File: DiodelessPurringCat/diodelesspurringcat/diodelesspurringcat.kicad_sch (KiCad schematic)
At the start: 21 parts, among them J1 ScreenL, U1 ProMicro-kbd

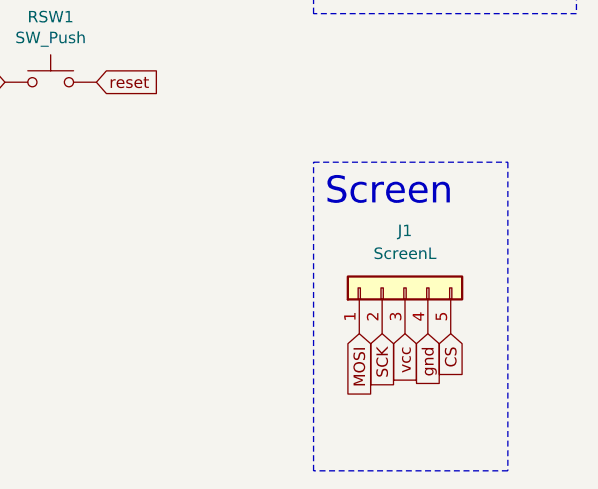
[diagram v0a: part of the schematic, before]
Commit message: trying to make a reversible nice view
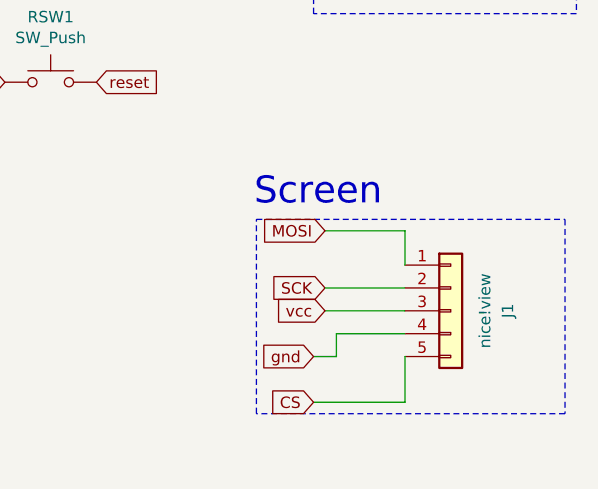
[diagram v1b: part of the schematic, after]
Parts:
- 0/9, 1/8, 10/19, 11/18, 12/17, 13/16, 14/15, 2/7, 20/25, 21/24, 22/23, 26/29, 27/28, 3/6, 4/5: footprint keyswitches:Kailh_socket_PG1350_reversible -> chelming-kbd:choc_v1_hotswap_reversible_no_extras
- J1: value ScreenL -> nice!view; footprint Connector_PinHeader_2.54mm:PinHeader_1x05_P2.54mm_Vertical -> chelming-kbd:nice-view_reversible
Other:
- moved on the sheet: J1
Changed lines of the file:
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@@
 	(polyline
 		(pts
-			(xy 227.33 124.46) (xy 205.74 124.46)
+			(xy 199.39 118.11) (xy 199.39 96.52)
 		)
 		(stroke
@@
 		)
 	)
+	(wire
+		(pts
+			(xy 205.74 111.76) (xy 208.28 111.76)
+		)
+		(stroke
+			(width 0)
+			(type default)
+		)
+	)
+	(wire
+		(pts
+			(xy 207.01 104.14) (xy 215.9 104.14)
+		)
+		(stroke
+			(width 0)
+			(type default)
+		)
+	)
+	(wire
+		(pts
+			(xy 205.74 116.84) (xy 215.9 116.84)
+		)
+		(stroke
+			(width 0)
+			(type default)
+		)
+	)
+	(wire
+		(pts
+			(xy 215.9 97.79) (xy 215.9 101.6)
+		)
+		(stroke
+			(width 0)
+			(type default)
+		)
+	)
+	(wire
+		(pts
+			(xy 215.9 116.84) (xy 215.9 111.76)
+		)
+		(stroke
+			(width 0)
+			(type default)
+		)
+	)
 	(polyline
 		(pts
-			(xy 227.33 90.17) (xy 227.33 124.46)
+			(xy 233.68 118.11) (xy 199.39 118.11)
 		)
 		(stroke
@@
 	(polyline
 		(pts
-			(xy 205.74 124.46) (xy 205.74 90.17)
+			(xy 199.39 96.52) (xy 233.68 96.52)
 		)
 		(stroke
@@
 	(polyline
 		(pts
-			(xy 205.74 90.17) (xy 227.33 90.17)
+			(xy 233.68 96.52) (xy 233.68 118.11)
 		)
 		(stroke
@@
 		)
 	)
+	(wire
+		(pts
+			(xy 208.28 109.22) (xy 215.9 109.22)
+		)
+		(stroke
+			(width 0)
+			(type default)
+		)
+	)
+	(wire
+		(pts
+			(xy 207.01 106.68) (xy 215.9 106.68)
+		)
+		(stroke
+			(width 0)
+			(type default)
+		)
+	)
+	(wire
+		(pts
+			(xy 208.28 111.76) (xy 208.28 109.22)
+		)
+		(stroke
+			(width 0)
+			(type default)
+		)
+	)
 	(polyline
 		(pts
@@
 		)
 	)
+	(wire
+		(pts
+			(xy 207.01 97.79) (xy 215.9 97.79)
+		)
+		(stroke
+			(width 0)
+			(type default)
+		)
+	)
 	(polyline
 		(pts
@@
 	(text "Screen"
 		(exclude_from_sim no)
-		(at 207.01 95.25 0)
+		(at 199.136 95.25 0)
 		(effects
 			(font
@@
 	(global_label "gnd"
 		(shape input)
-		(at 218.44 109.22 270)
-		(fields_autoplaced yes)
-		(effects
-			(font
-				(size 1.27 1.27)
-			)
-			(justify right)
-		)
-		(property "Intersheetrefs" "${INTERSHEET_REFS}"
-			(at 218.3606 114.9913 90)
+		(at 205.74 111.76 180)
+		(fields_autoplaced yes)
+		(effects
+			(font
+				(size 1.27 1.27)
+			)
+			(justify right)
+		)
+		(property "Intersheetrefs" "${INTERSHEET_REFS}"
+			(at 199.962 111.76 0)
 			(effects
 				(font
@@
 	(global_label "CS"
 		(shape input)
-		(at 220.98 109.22 270)
-		(fields_autoplaced yes)
-		(effects
-			(font
-				(size 1.27 1.27)
-			)
-			(justify right)
-		)
-		(property "Intersheetrefs" "${INTERSHEET_REFS}"
-			(at 220.9006 114.0237 90)
+		(at 205.74 116.84 180)
+		(fields_autoplaced yes)
+		(effects
+			(font
+				(size 1.27 1.27)
+			)
+			(justify right)
+		)
+		(property "Intersheetrefs" "${INTERSHEET_REFS}"
+			(at 200.9295 116.84 0)
 			(effects
 				(font
@@
 	(global_label "vcc"
 		(shape input)
-		(at 215.9 109.22 270)
-		(fields_autoplaced yes)
-		(effects
-			(font
-				(size 1.27 1.27)
-			)
-			(justify right)
-		)
-		(property "Intersheetrefs" "${INTERSHEET_REFS}"
-			(at 215.8206 114.689 90)
+		(at 207.01 106.68 180)
+		(fields_autoplaced yes)
+		(effects
+			(font
+				(size 1.27 1.27)
+			)
+			(justify right)
+		)
+		(property "Intersheetrefs" "${INTERSHEET_REFS}"
+			(at 201.5342 106.68 0)
 			(effects
 				(font
@@
 	(global_label "SCK"
 		(shape input)
-		(at 213.36 109.22 270)
-		(fields_autoplaced yes)
-		(effects
-			(font
-				(size 1.27 1.27)
-			)
-			(justify right)
-		)
-		(property "Intersheetrefs" "${INTERSHEET_REFS}"
-			(at 213.2806 115.2937 90)
+		(at 207.01 104.14 180)
+		(fields_autoplaced yes)
+		(effects
+			(font
+				(size 1.27 1.27)
+			)
+			(justify right)
+		)
+		(property "Intersheetrefs" "${INTERSHEET_REFS}"
+			(at 200.9295 104.14 0)
 			(effects
 				(font
@@
 	(global_label "MOSI"
 		(shape input)
-		(at 210.82 109.22 270)
-		(fields_autoplaced yes)
-		(effects
-			(font
-				(size 1.27 1.27)
-			)
-			(justify right)
-		)
-		(property "Intersheetrefs" "${INTERSHEET_REFS}"
-			(at 210.7406 116.1404 90)
+		(at 207.01 97.79 180)
+		(fields_autoplaced yes)
+		(effects
+			(font
+				(size 1.27 1.27)
+			)
+			(justify right)
+		)
+		(property "Intersheetrefs" "${INTERSHEET_REFS}"
+			(at 200.0828 97.79 0)
 			(effects
 				(font
@@
 			)
 		)
-		(property "Footprint" "keyswitches:Kailh_socket_PG1350_reversible"
+		(property "Footprint" "chelming-kbd:choc_v1_hotswap_reversible_no_extras"
 			(at 26.67 33.02 0)
 			(effects
@@
 			)
 		)
-		(property "Footprint" "keyswitches:Kailh_socket_PG1350_reversible"
+		(property "Footprint" "chelming-kbd:choc_v1_hotswap_reversible_no_extras"
 			(at 49.53 24.13 0)
 			(effects
@@
 			)
 		)
-		(property "Footprint" "keyswitches:Kailh_socket_PG1350_reversible"
+		(property "Footprint" "chelming-kbd:choc_v1_hotswap_reversible_no_extras"
 			(at 72.39 20.32 0)
 			(effects
@@
 			)
 		)
-		(property "Footprint" "keyswitches:Kailh_socket_PG1350_reversible"
+		(property "Footprint" "chelming-kbd:choc_v1_hotswap_reversible_no_extras"
 			(at 95.25 24.13 0)
 			(effects
@@
 			)
 		)
-		(property "Footprint" "keyswitches:Kailh_socket_PG1350_reversible"
+		(property "Footprint" "chelming-kbd:choc_v1_hotswap_reversible_no_extras"
 			(at 95.25 86.36 0)
 			(effects
@@
 			)
 		)
-		(property "Footprint" "keyswitches:Kailh_socket_PG1350_reversible"
+		(property "Footprint" "chelming-kbd:choc_v1_hotswap_reversible_no_extras"
 			(at 26.67 54.61 0)
 			(effects
@@
 			)
 		)
-		(property "Footprint" "keyswitches:Kailh_socket_PG1350_reversible"
+		(property "Footprint" "chelming-kbd:choc_v1_hotswap_reversible_no_extras"
 			(at 49.53 45.72 0)
 			(effects
@@
 			)
 		)
-		(property "Footprint" "keyswitches:Kailh_socket_PG1350_reversible"
+		(property "Footprint" "chelming-kbd:choc_v1_hotswap_reversible_no_extras"
 			(at 72.39 41.91 0)
 			(effects
@@
 			)
 		)
-		(property "Footprint" "keyswitches:Kailh_socket_PG1350_reversible"
+		(property "Footprint" "chelming-kbd:choc_v1_hotswap_reversible_no_extras"
 			(at 95.25 45.72 0)
 			(effects
@@
 			)
 		)
-		(property "Footprint" "keyswitches:Kailh_socket_PG1350_reversible"
+		(property "Footprint" "chelming-kbd:choc_v1_hotswap_reversible_no_extras"
 			(at 49.53 64.77 0)
 			(effects
@@
 			)
 		)
-		(property "Footprint" "keyswitches:Kailh_socket_PG1350_reversible"
+		(property "Footprint" "chelming-kbd:choc_v1_hotswap_reversible_no_extras"
 			(at 72.39 60.96 0)
 			(effects
@@
 			)
 		)
-		(property "Footprint" "keyswitches:Kailh_socket_PG1350_reversible"
+		(property "Footprint" "chelming-kbd:choc_v1_hotswap_reversible_no_extras"
 			(at 95.25 64.77 0)
 			(effects
@@
 			)
 		)
-		(property "Footprint" "keyswitches:Kailh_socket_PG1350_reversible"
+		(property "Footprint" "chelming-kbd:choc_v1_hotswap_reversible_no_extras"
 			(at 118.11 34.29 0)
 			(effects
@@
 			)
 		)
-		(property "Footprint" "keyswitches:Kailh_socket_PG1350_reversible"
+		(property "Footprint" "chelming-kbd:choc_v1_hotswap_reversible_no_extras"
 			(at 118.11 55.88 0)
 			(effects
@@
 	(symbol
 		(lib_id "Connector_Generic:Conn_01x05")
-		(at 215.9 104.14 90)
+		(at 220.98 106.68 0)
 		(unit 1)
 		(exclude_from_sim no)
@@
 		(fields_autoplaced yes)
 		(property "Reference" "J1"
-			(at 215.9 97.79 90)
-			(effects
-				(font
-					(size 1.27 1.27)
-				)
-			)
-		)
-		(property "Value" "ScreenL"
-			(at 215.9 100.33 90)
-			(effects
-				(font
-					(size 1.27 1.27)
-				)
-			)
-		)
-		(property "Footprint" "Connector_PinHeader_2.54mm:PinHeader_1x05_P2.54mm_Vertical"
-			(at 215.9 104.14 0)
+			(at 227.33 106.68 90)
+			(effects
+				(font
+					(size 1.27 1.27)
+				)
+			)
+		)
+		(property "Value" "nice!view"
+			(at 224.79 106.68 90)
+			(effects
+				(font
+					(size 1.27 1.27)
+				)
+			)
+		)
+		(property "Footprint" "chelming-kbd:nice-view_reversible"
+			(at 220.98 106.68 0)
 			(effects
 				(font
@@
 		)
 		(property "Datasheet" "~"
-			(at 215.9 104.14 0)
+			(at 220.98 106.68 0)
 			(effects
 				(font
@@
 		)
 		(property "Description" ""
-			(at 215.9 104.14 0)
+			(at 220.98 106.68 0)
 			(effects
 				(font
@@
 			)
 		)
-		(property "Footprint" "keyswitches:Kailh_socket_PG1350_reversible"
+		(property "Footprint" "chelming-kbd:choc_v1_hotswap_reversible_no_extras"
 			(at 118.11 86.36 0)
 			(effects
